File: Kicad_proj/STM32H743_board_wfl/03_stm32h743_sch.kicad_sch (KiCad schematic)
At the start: 35 parts, among them J1 GPS, J2 ESC, J3 UART, J4 Tag_Connect_6pin, U3 STM32H743VITx, U4 W25Q512JVEIQ, Y1 TSX-3225_16.0000MF18X-AC0

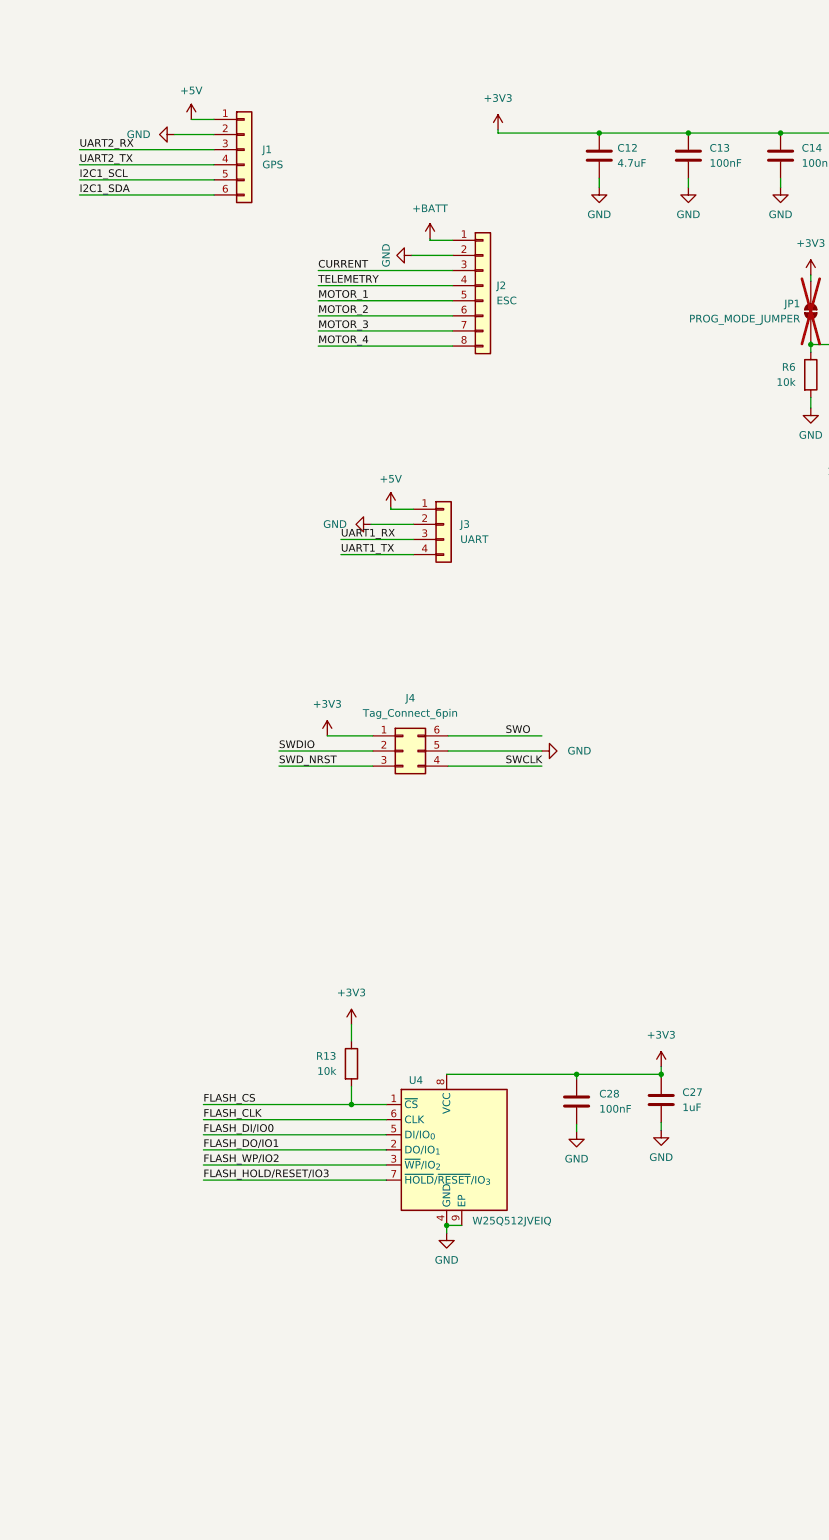
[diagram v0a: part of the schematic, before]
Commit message: PCB v1.0
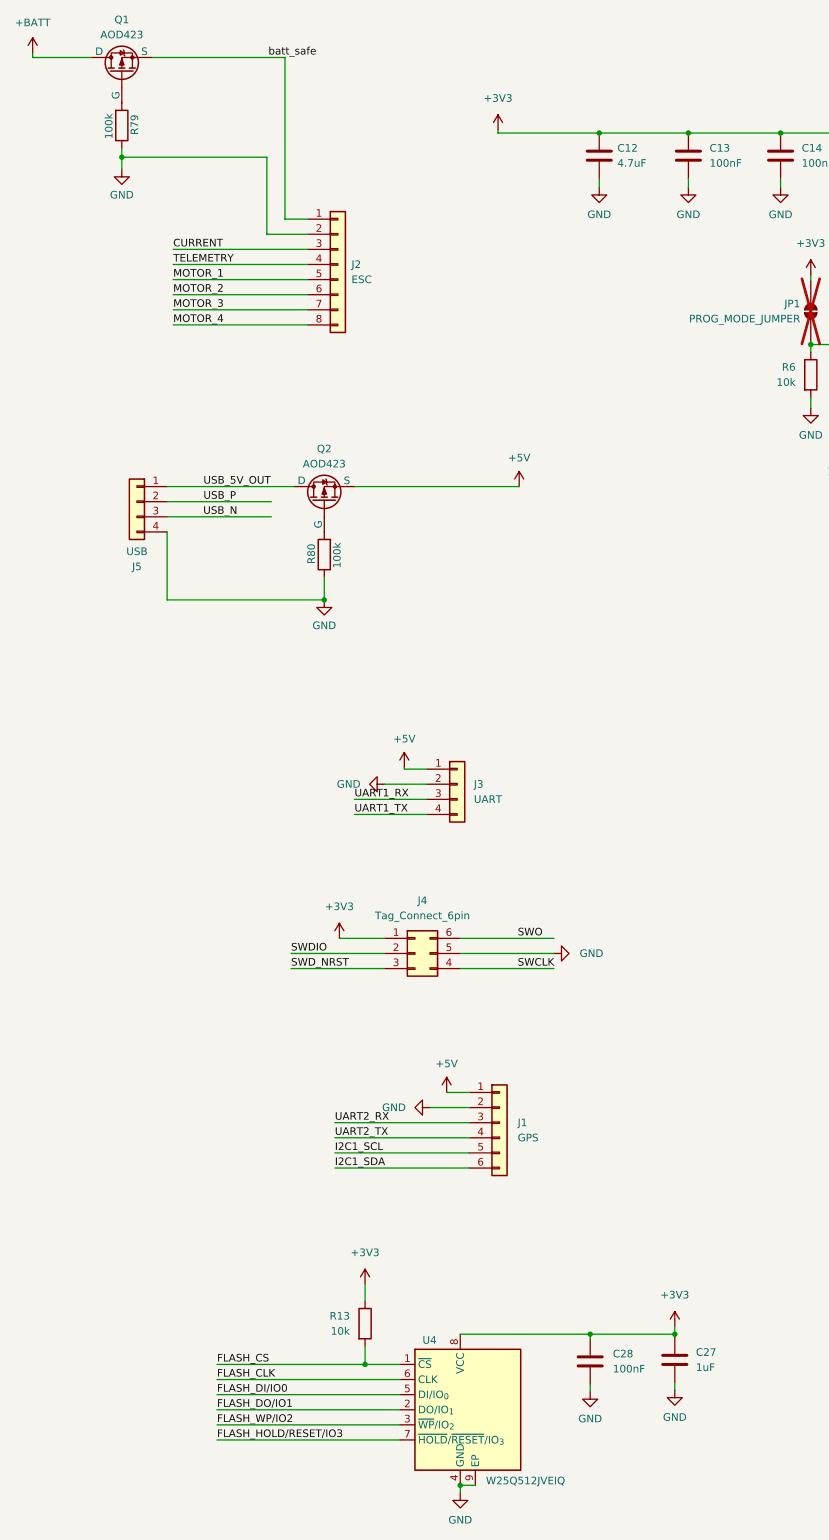
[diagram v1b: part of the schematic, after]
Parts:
- added J5: USB, Connector_JST:JST_GH_SM04B-GHS-TB_1x04-1MP_P1.25mm_Horizontal, symbol Connector_Generic:Conn_01x04
- added Q1, Q2: AOD423, wfl_lib:TO-252-2_AOD423, symbol WFL_SYMBOL_LIB_KICAD:AOD423
- added R79, R80: 100k, Resistor_SMD:R_0603_1608Metric_Pad0.98x0.95mm_HandSolder, symbol Device:R
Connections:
- net +5V: now also Q2.3 (S)
- net +BATT: now also Q1.2 (D); no longer J2.1 (Pin_1)
- net GND: now also J5.4 (Pin_4), R79.1, R80.1
- new net: Q2.1 (G), R80.2
- new net: Q1.1 (G), R79.2
- new net USB_5V_OUT: J5.1 (Pin_1), Q2.2 (D)
- new net USB_N: J5.3 (Pin_3)
- new net USB_P: J5.2 (Pin_2)
- new net batt_safe: J2.1 (Pin_1), Q1.3 (S)
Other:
- moved on the sheet: C27, C28, J1, J2, J3, J4, R13, U4
